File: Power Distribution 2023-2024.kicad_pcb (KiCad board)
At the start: 2 copper layers, 53.3 x 55.2 mm, 29 parts, among them J1 TEL_OUT, J2 STEER_OUT, J3 SAFE_OUT, J4 12V_IN, J5 L_KILL, J6 R_KILL, J7 SAFE_KILL

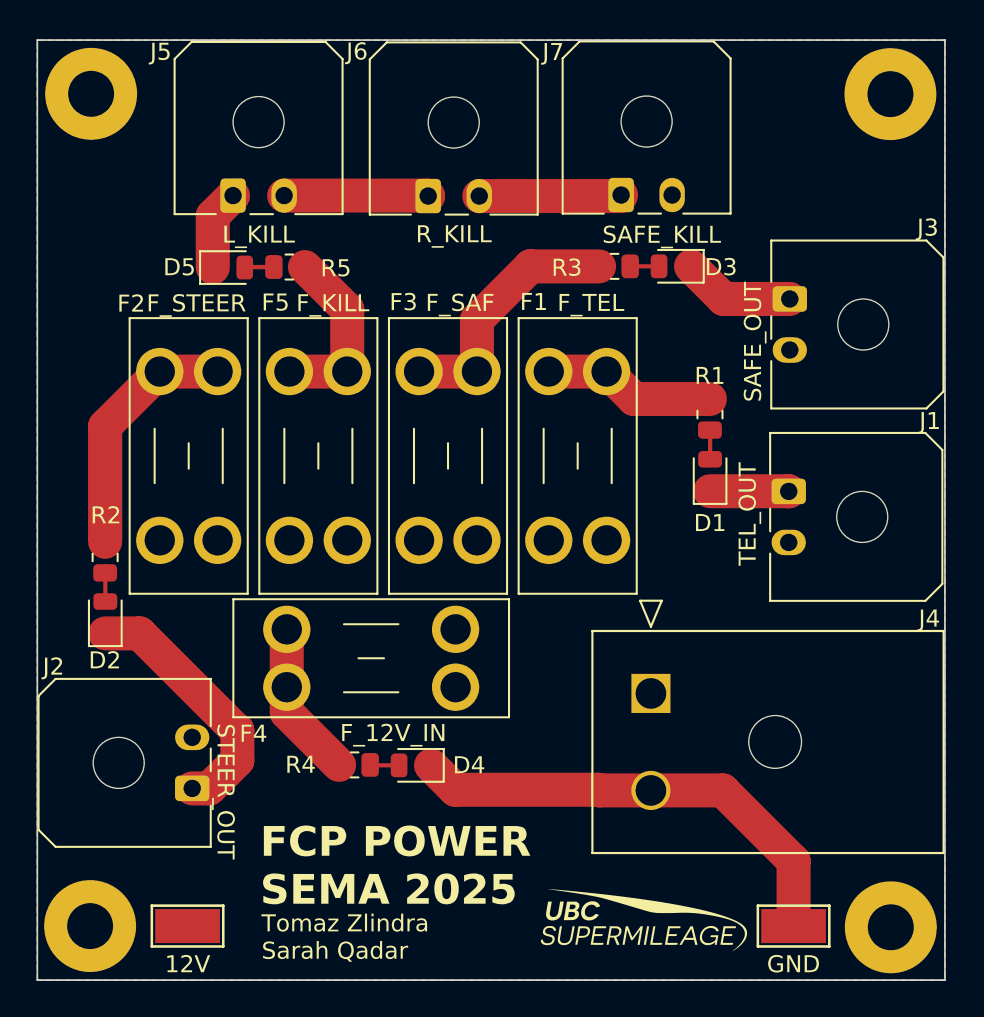
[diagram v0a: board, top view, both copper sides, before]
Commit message: cleaned up stuff
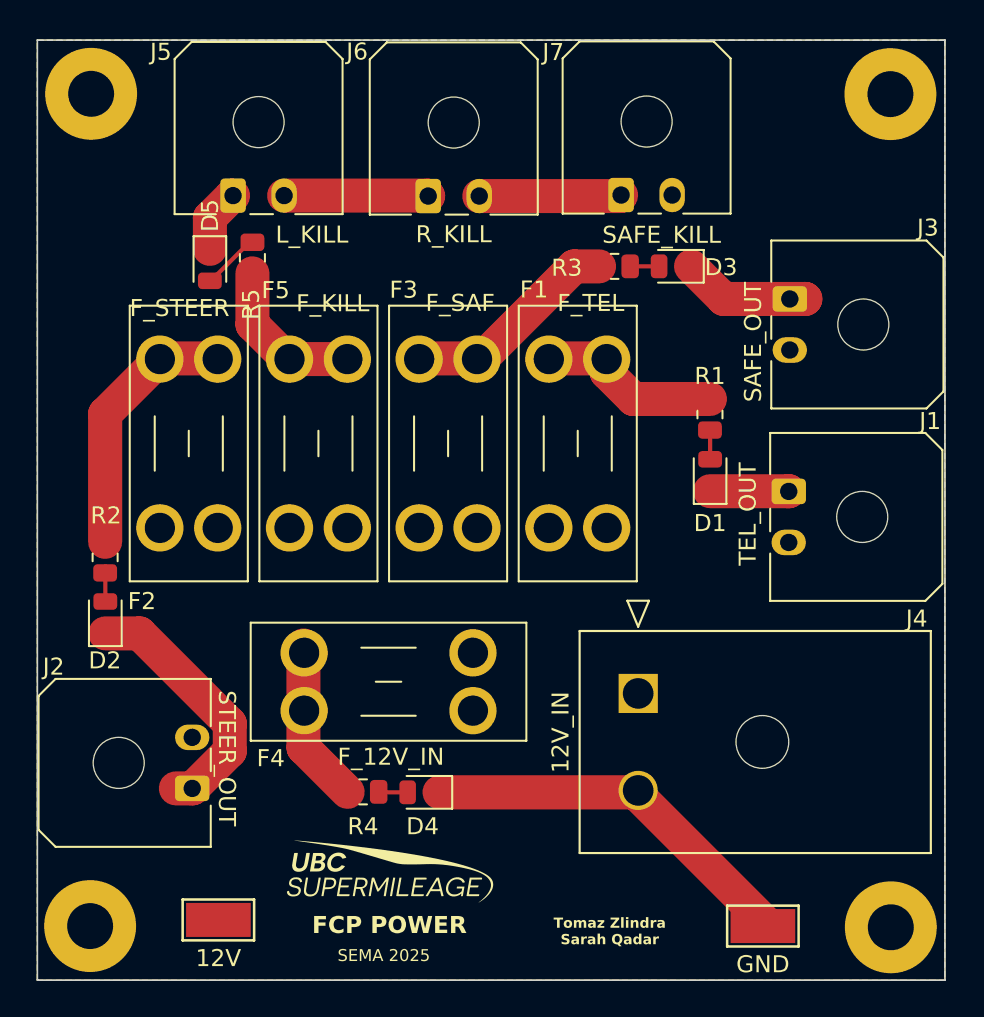
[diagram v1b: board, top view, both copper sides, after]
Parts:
- moved G*** 15.2 mm to (234.0, 147.0)
- moved R5 2.24 mm to (226.0, 110.6), turned to 90 degrees
- moved REF** 1.85 mm to (224.0, 149.5)
- moved REF** 1.80 mm to (256.0, 149.9)
- moved F4 1.72 mm to (229.0, 133.8)
- moved D4 1.66 mm to (236.1, 142.0)
- moved R4 1.66 mm to (232.5, 142.0)
- moved D5 1.12 mm to (223.5, 111.0), turned to -90 degrees
- moved J4 0.75 mm to (248.7, 136.2)
- moved F2 0.73 mm to (220.6, 126.5)
- moved F3 0.73 mm to (235.8, 126.5)
- moved F5 0.73 mm to (228.2, 126.5)
- moved F1 0.73 mm to (243.4, 126.5)
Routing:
- net GND: track 27.5 -> 22.9 mm
- net Net-(F3-Pad2): track 15.5 -> 13.4 mm
- net Net-(D5-A): track 1.72 -> 3.44 mm
- net Net-(F5-Pad2): track 10.8 -> 9.54 mm
- net Net-(D5-K): track 4.73 -> 3.73 mm
- net Net-(D3-K): track 6.61 -> 7.53 mm
- net Net-(F2-Pad2): track 14.7 -> 15.5 mm
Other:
- board text added: "FCP POWER"
- board text added: "SEMA 2025"
- board text removed: "FCP POWER SEMA 2025"

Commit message: FINAL for printing (unless there are any last changes)
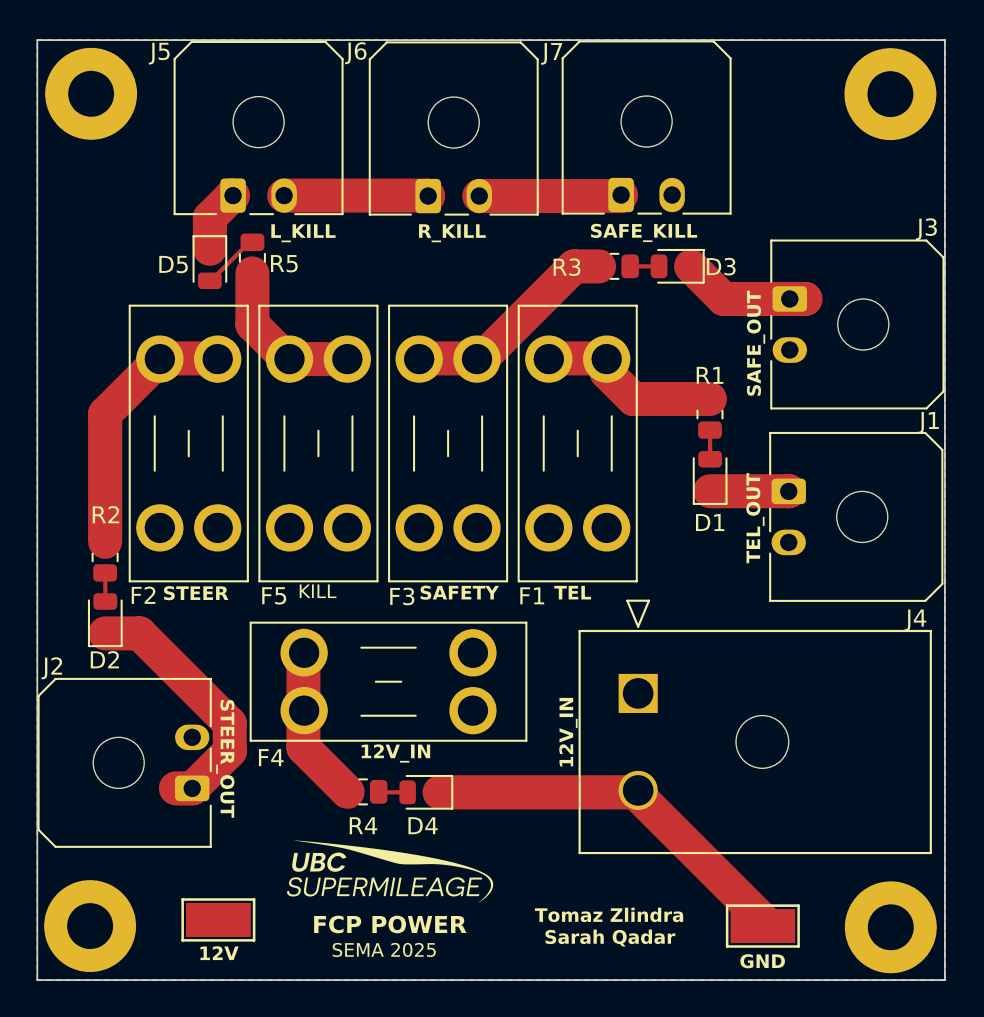
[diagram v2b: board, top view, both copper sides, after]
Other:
- board text added: "12V_IN"
- board text added: "KILL"
- board text added: "SAFETY"
- board text added: "STEER"
- board text added: "TEL"
- board text removed: "F_12V_IN"
- board text removed: "F_KILL"
- board text removed: "F_SAF"
- board text removed: "F_STEER"
- board text removed: "F_TEL"
